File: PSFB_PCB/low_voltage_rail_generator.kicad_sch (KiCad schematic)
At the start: 27 parts, among them IC11 TPS561246DRLR, IC4 UA78M05CDCYG3, J1 12V_Jumper_for_5V, J24 5V_PIN_IN_DEBUG, J4 3.3V_PIN_IN_DEBUG, J7 Power_Terminal_12V, J8 12V_Jumper_for_3.3V, U3 SN6507DGQ

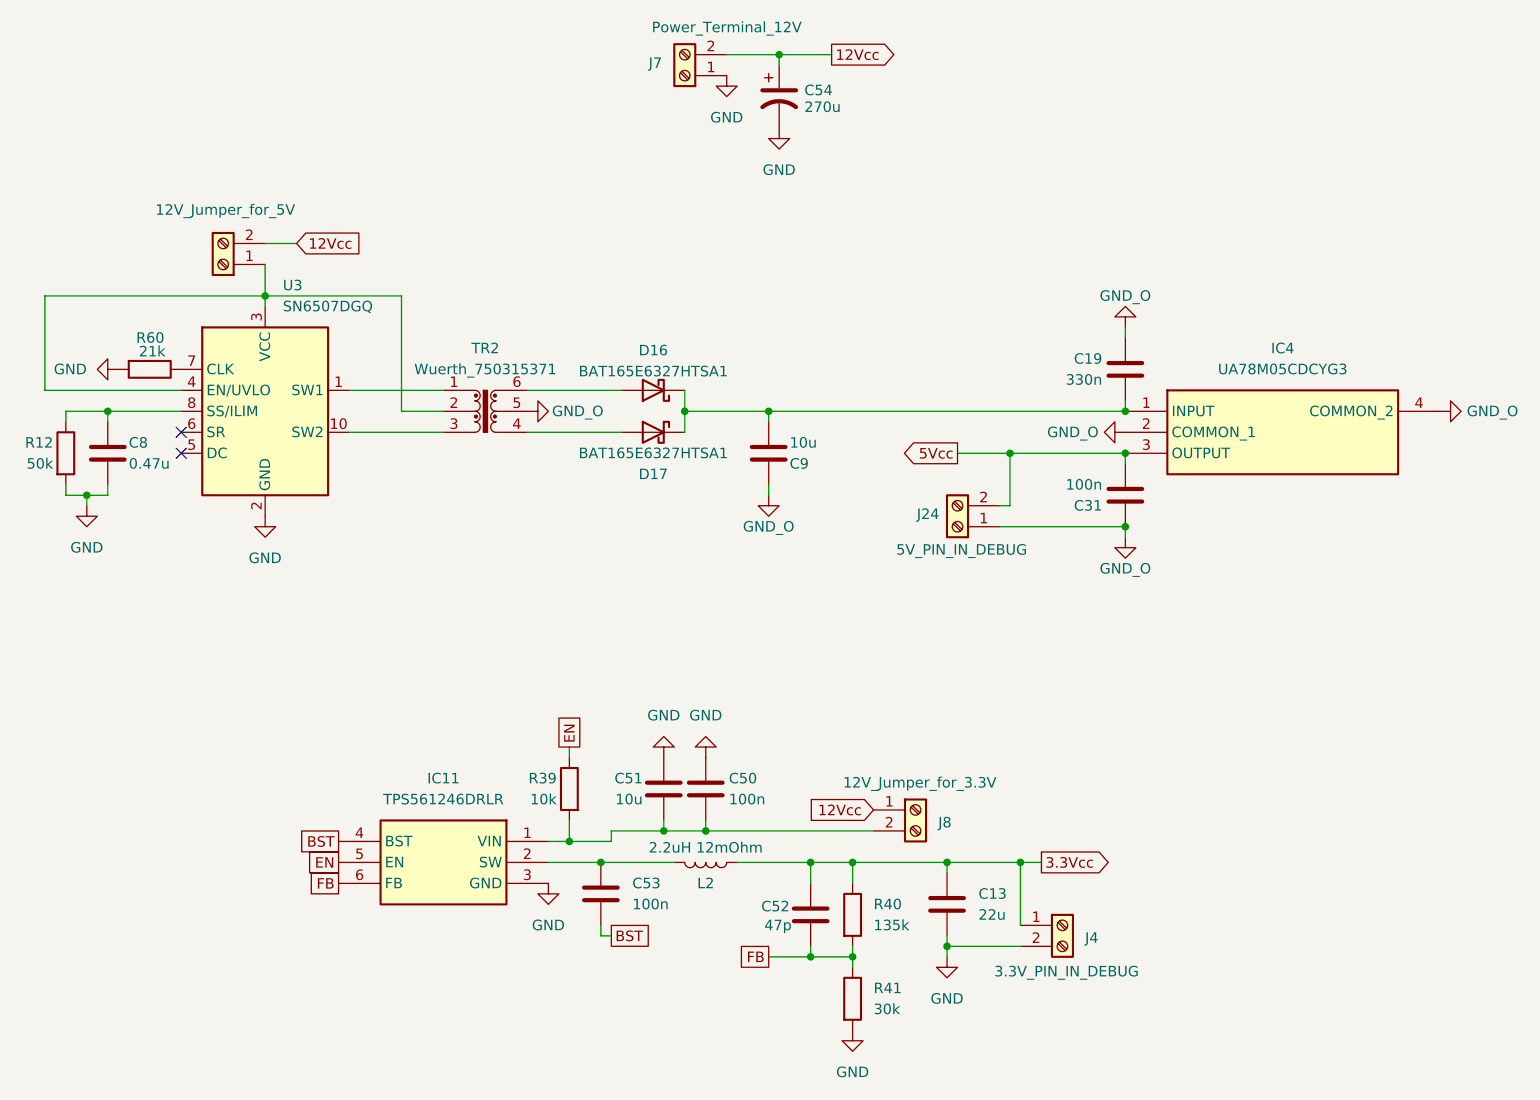
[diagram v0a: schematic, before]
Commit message: updating Work
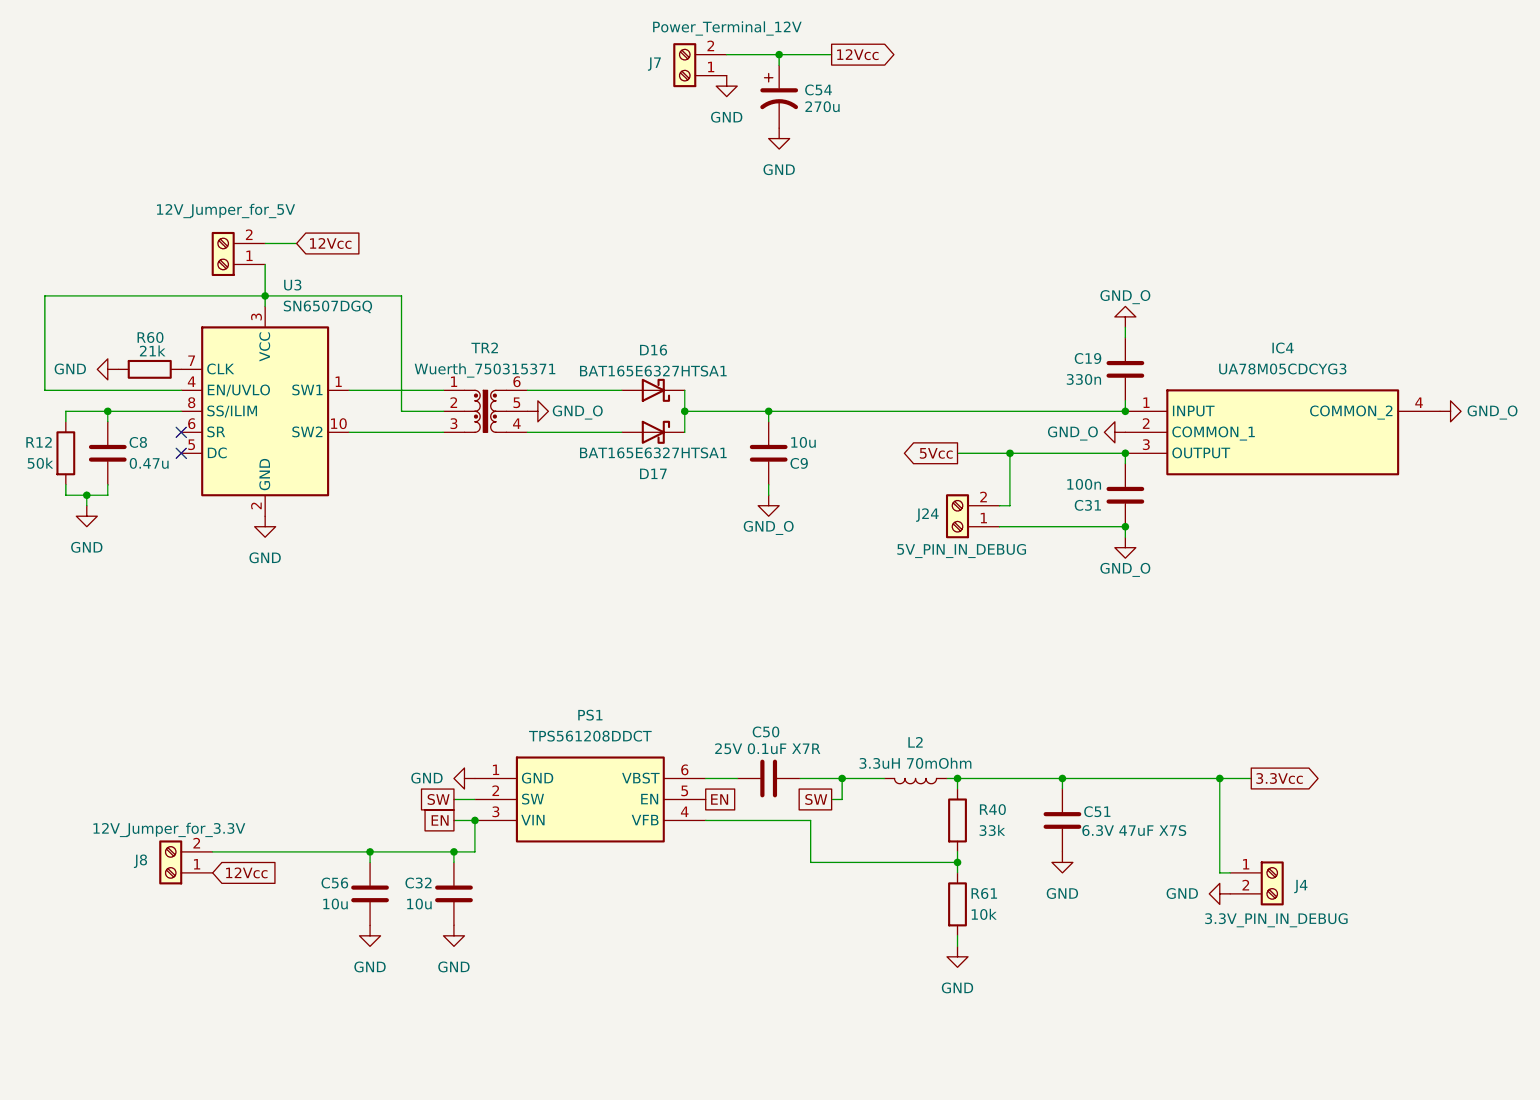
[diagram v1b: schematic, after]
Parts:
- removed C13: 22u, Capacitor_SMD:C_1206_3216Metric, symbol Device:C
- removed C52: 47p, Capacitor_SMD:C_0603_1608Metric_Pad1.08x0.95mm_HandSolder, symbol Device:C
- removed C53: 100n, Capacitor_SMD:C_1812_4532Metric, symbol Device:C
- removed IC11: TPS561246DRLR, oscar:SOTFL50P160X60-6N, symbol oscar:TPS561246DRLR
- removed R39: 10k, Resistor_SMD:R_0603_1608Metric_Pad0.98x0.95mm_HandSolder, symbol Device:R
- removed R41: 30k, Resistor_SMD:R_0603_1608Metric_Pad0.98x0.95mm_HandSolder, symbol Device:R
- added C32, C56: 10u, Capacitor_SMD:C_1206_3216Metric, symbol Device:C
- added PS1: TPS561208DDCT, SOT95P280X110-6N, symbol oscar:TPS561208DDCT
- added R61: 10k, Resistor_SMD:R_0603_1608Metric_Pad0.98x0.95mm_HandSolder, symbol Device:R
- C50: value 100n -> 25V 0.1uF X7R; footprint Capacitor_SMD:C_1206_3216Metric_Pad1.33x1.80mm_HandSolder -> Capacitor_SMD:C_0805_2012Metric_Pad1.18x1.45mm_HandSolder
- C51: value 10u -> 6.3V 47uF X7S; footprint Capacitor_SMD:C_1206_3216Metric -> Capacitor_SMD:C_1206_3216Metric_Pad1.33x1.80mm_HandSolder
- L2: value 2.2uH 12mOhm -> 3.3uH 70mOhm; footprint oscar:WE-LHMI_7030_705048 -> oscar:784777033
- R40: value 135k -> 33k
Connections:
- net 3.3Vcc: now also C51.1
- net EN: now also J8.2 (Pin_2), C32.1, C56.1, PS1.3 (VIN), PS1.5 (EN)
- net GND: now also C51.2, C32.2, C56.2, PS1.1 (GND), R61.2; no longer C50.1, C51.1
- net SW: now reaches L2.2
- net SW: now also C50.1, PS1.2 (SW)
- net FB: no longer names the net of R40.2
- net FB: now also PS1.4 (VFB), R61.1
- new net: C50.2, PS1.6 (VBST)
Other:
- moved on the sheet: C50, J4, J8, L2, R40
